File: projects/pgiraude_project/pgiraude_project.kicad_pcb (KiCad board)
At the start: 2 copper layers, 17 parts, among them SW1 SW_Push, Y1 16MHz

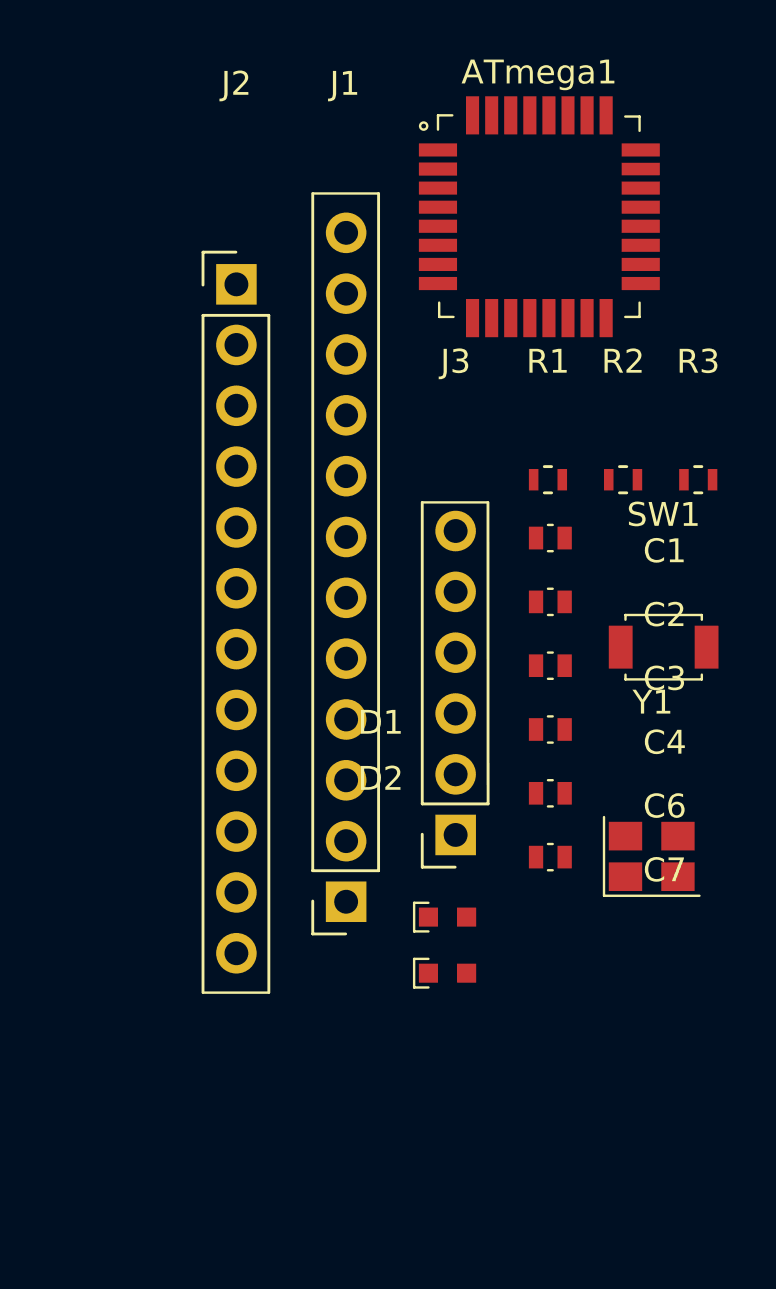
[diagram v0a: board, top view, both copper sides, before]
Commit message: last
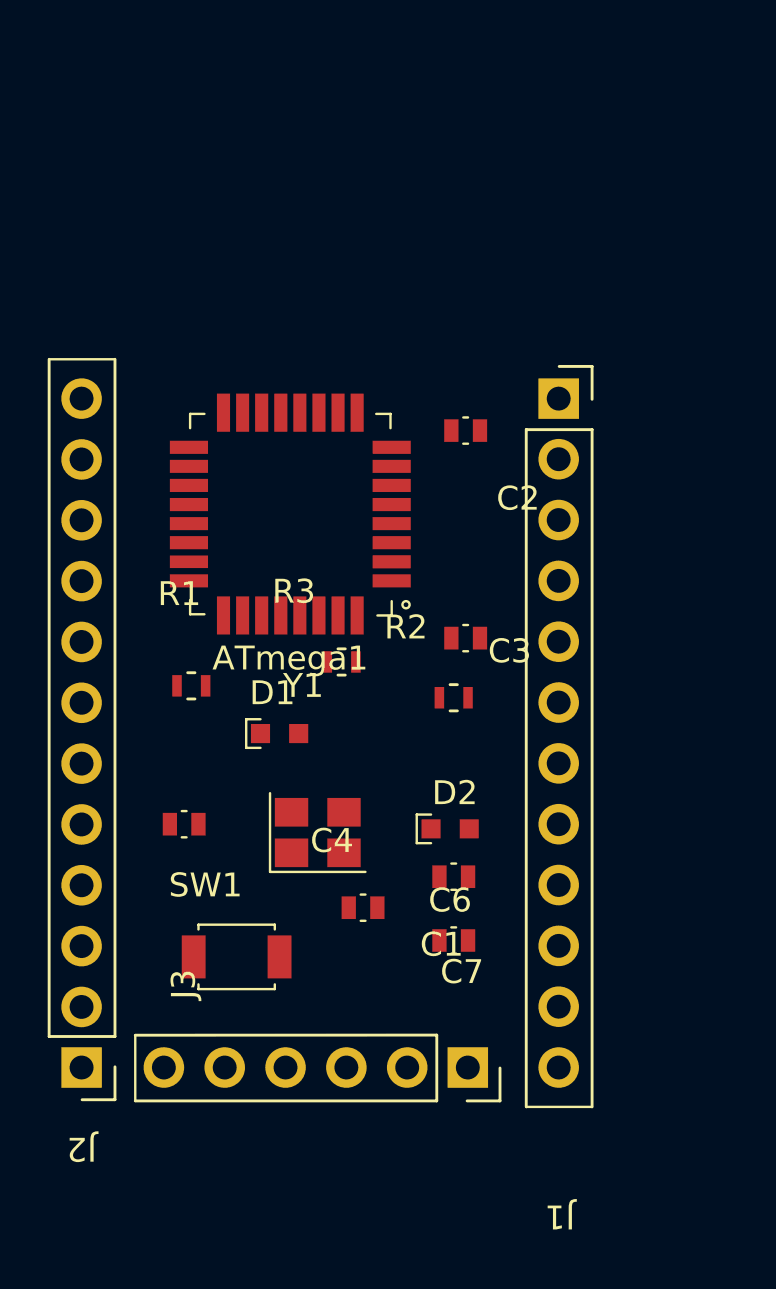
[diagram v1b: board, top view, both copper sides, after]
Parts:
- moved J2 49.1 mm to (70.0, 124.4), turned to 180 degrees
- moved J1 47.4 mm to (90.0, 122.2), turned to 180 degrees
- moved J3 34.7 mm to (66.8, 116.5), turned to 90 degrees
- moved SW1 22.1 mm to (76.5, 106.8)
- moved C1 17.4 mm to (82.5, 110.5)
- moved R1 17.3 mm to (74.6, 96.0)
- moved R3 16.8 mm to (80.9, 95.0)
- moved ATmega1 16.3 mm to (78.8, 93.3), turned to 180 degrees
- moved C4 15.9 mm to (75.0, 107.0)
- moved Y1 14.0 mm to (80.0, 100.7)
- moved R2 11.6 mm to (85.6, 96.5)
- moved D1 10.4 mm to (78.3, 102.5)
- moved C2 8.01 mm to (86.8, 90.5)
- moved D2 6.05 mm to (85.5, 106.5)
- moved C6 5.35 mm to (86.3, 109.2)
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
